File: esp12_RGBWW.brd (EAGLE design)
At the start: 49.5 x 50.5 mm, 24 parts

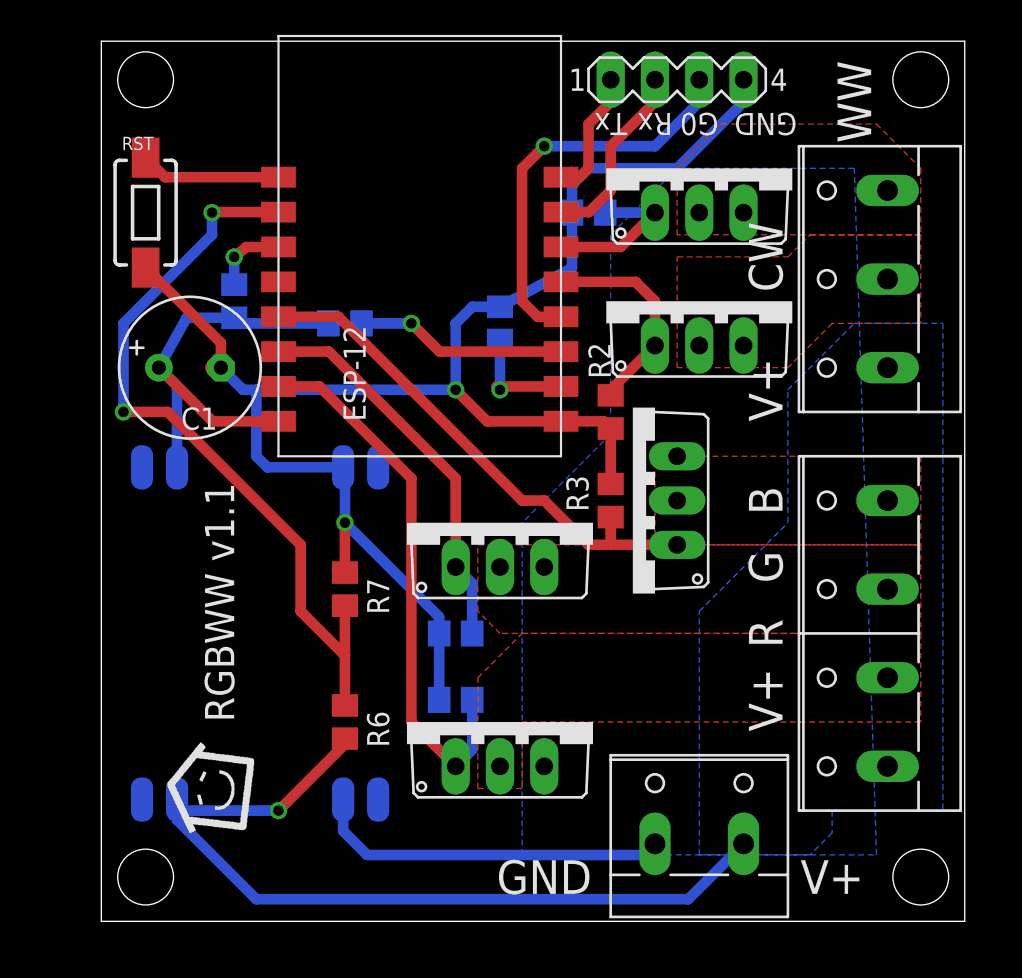
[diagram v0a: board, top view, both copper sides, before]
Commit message: v1.2
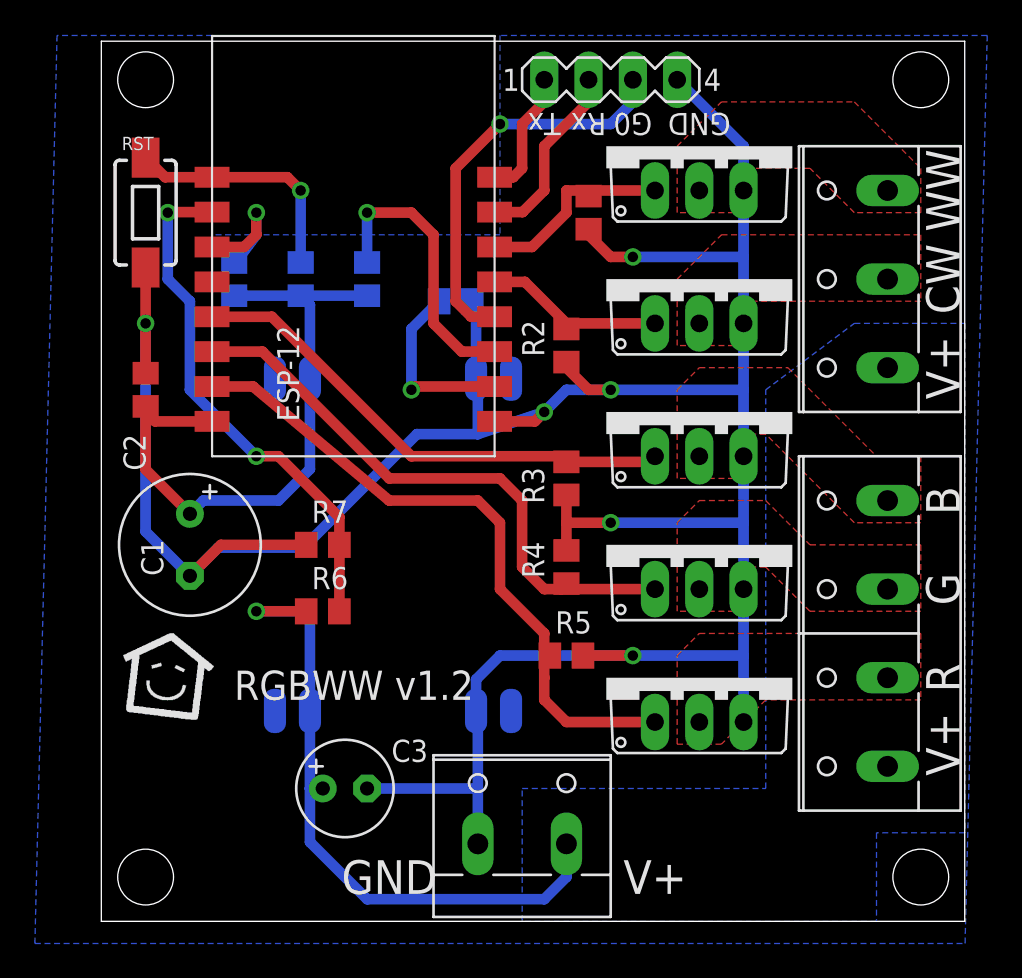
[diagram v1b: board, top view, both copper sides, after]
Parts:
- added C2: 100n, rcl:C0805
- added C3: (no value), resistor:E2,5-6
- added REST: 10k, rcl:R0805
- moved IRLZ44N-R 11.7 mm to (34.3, 14.0)
- moved IRLZ44N-G 11.5 mm to (34.3, 21.6)
- moved C1 10.2 mm to (5.08, 21.6), turned to 270 degrees
- moved VCC 10.2 mm to (24.1, 5.08)
- moved U$1 9.92 mm to (1.27, 11.4), turned to 0 degrees
- moved DC_CONVERTER 9.16 mm to (16.5, 21.6)
- moved R4 7.41 mm to (26.7, 20.3), flipped to the top, turned to 90 degrees
- moved R5 6.84 mm to (26.7, 15.2), flipped to the top
- moved R6 6.48 mm to (12.7, 17.8), turned to 180 degrees
- moved IRLZ44N-B 6.35 mm to (34.3, 29.2), turned to 0 degrees
- moved R2 4.58 mm to (26.7, 33.0)
- moved PROG 3.81 mm to (29.2, 48.3)
- moved ESP-12 3.81 mm to (6.35, 26.7)
- moved GPIO15 2.84 mm to (20.3, 35.6), turned to 180 degrees
- moved R7 2.84 mm to (12.7, 21.6), turned to 0 degrees
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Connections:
- removed net GND3.3V: C1.-, DC_CONVERTER.OUT-(2), ESP-12.1, GPIO15.2, PROG.4, R1.1, R2.2, R3.2, R4.2, R5.2, R7.1, RST.1
- removed net N$20: C1.+, CH_PD.2, DC_CONVERTER.OUT+(1), ESP-12.16, GPIO2.2
- new net +3V3: C1.+, C2.2, CH_PD.2, DC_CONVERTER.OUT+(1), ESP-12.16, GPIO2.2, REST.1
- net +12V: now also C3.+
- net GND: now also C1.-, C2.1, C3.-, DC_CONVERTER.OUT-(2), ESP-12.1, GPIO15.2, PROG.4, R1.1, R2.2, R3.2, R4.2, R5.2, R7.1, RST.1
- net N$12: now also REST.2
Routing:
- net GND: track 20.5 -> 175.1 mm, vias 0 -> 6
- net GND3.3V: track 91.8 -> 0.00 mm, vias 2 -> 0
- net +3V3: track 0.00 -> 37.5 mm
- net N$20: track 25.8 -> 0.00 mm
- net N$21: track 43.8 -> 30.2 mm
- net R4: track 22.5 -> 33.7 mm
- net +12V: track 48.4 -> 38.1 mm
- net N$23: track 31.6 -> 38.4 mm
- net N$12: track 8.08 -> 13.8 mm, vias 0 -> 1
- net N$3: track 12.1 -> 16.4 mm
- net N$7: track 6.82 -> 10.6 mm
- net N$2: track 4.33 -> 7.41 mm
- net N$25: track 9.07 -> 11.6 mm
- net N$24: track 12.3 -> 10.6 mm
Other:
- board text added: "RGBWW v1.2"
- board text removed: "RGBWW v1.1"
